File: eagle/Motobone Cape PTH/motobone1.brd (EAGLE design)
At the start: 87.3 x 54.6 mm, 23 parts, among them J1 COMPUTER-PERIPHERAL-POWERRA

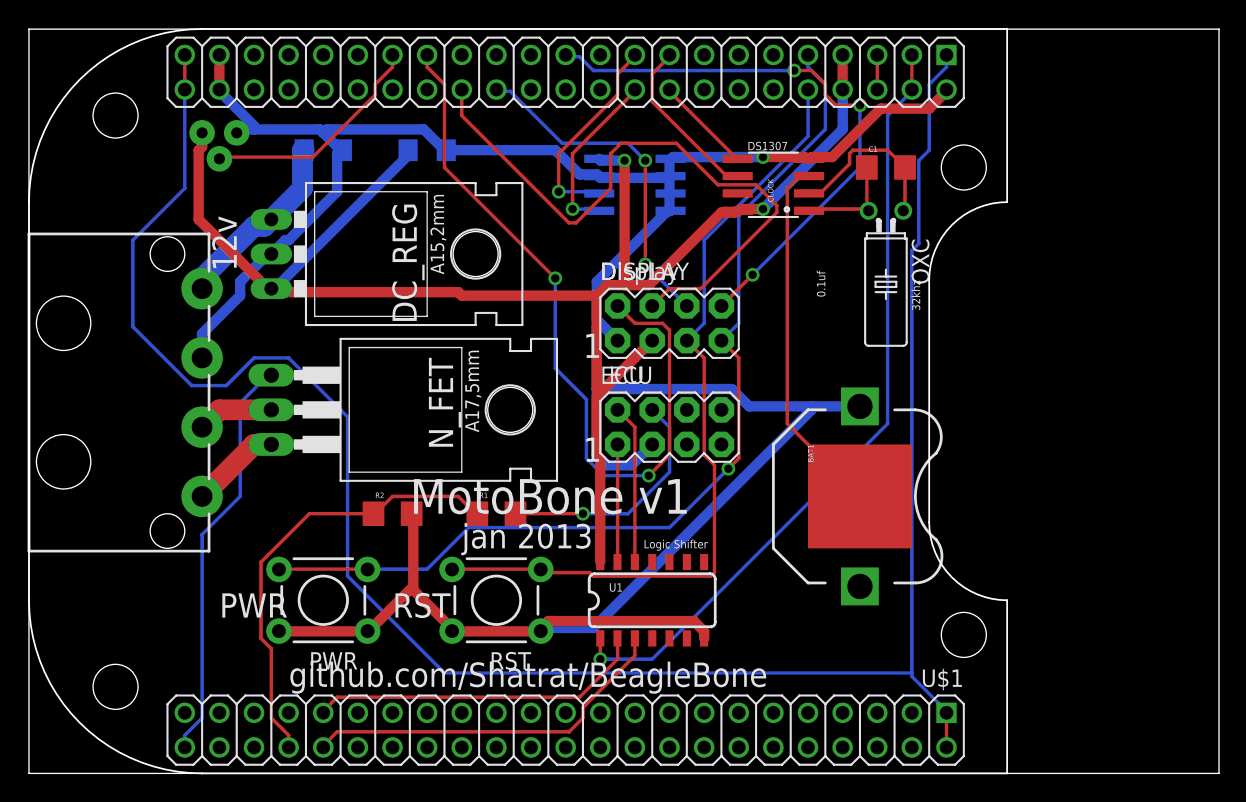
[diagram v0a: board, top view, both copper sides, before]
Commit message: updating Eagle files
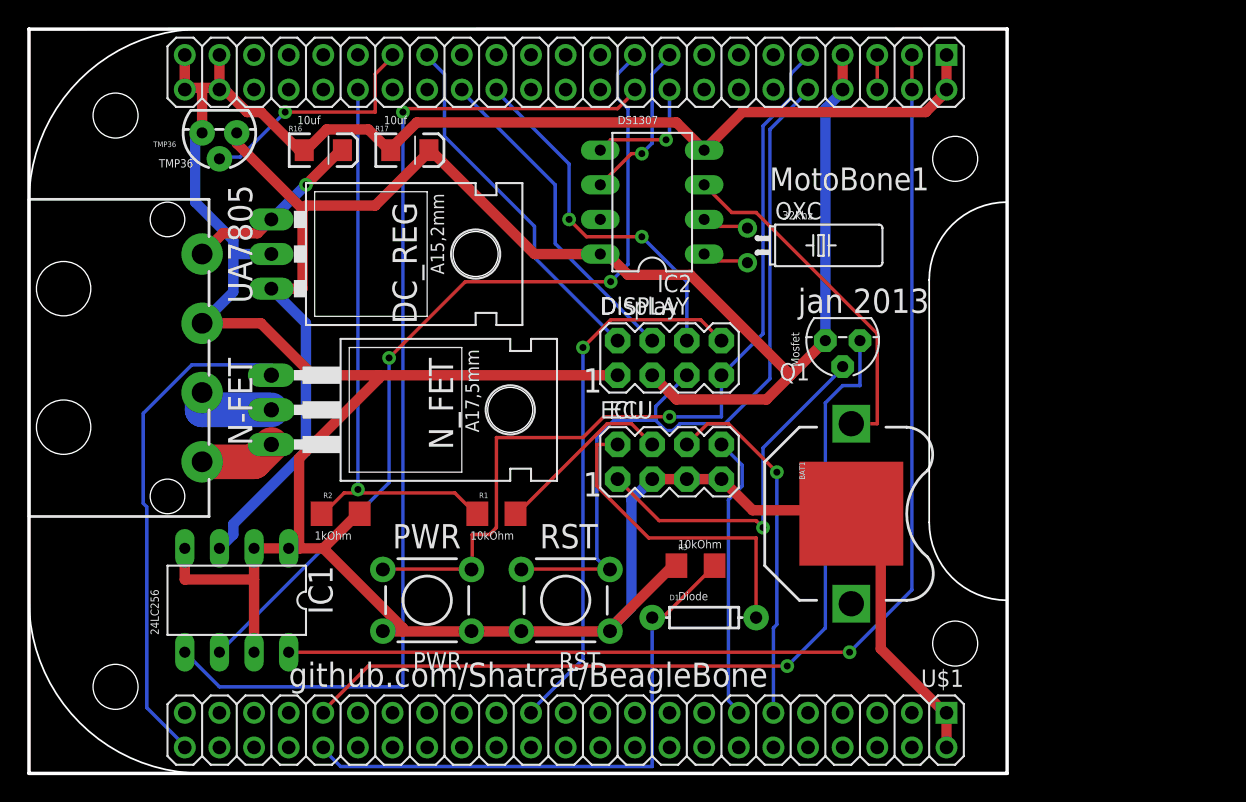
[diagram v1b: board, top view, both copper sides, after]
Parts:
- removed C1: 0.1uF, SparkFun-Capacitors:1206
- removed CLOCK: DS1307SO8, SparkFun-FreqCtrl:SO08
- removed EEPROM: EEPROM-I2CSMD, SparkFun-DigitalIC:SO08
- removed U1: (no value), SparkFun-DigitalIC:SO14
- added D1: (no value), SparkFun-DiscreteSemi:DIODE-1N4148
- added IC1: 24LC256P, microchip:DIL8
- added IC2: DS1307, adafruit:DIL08
- added Q1: FQN1N50C, adafruit:TO92
- added R3: 10k, SparkFun-Resistors:1206
- BAT1: value (none) -> 3v
- R2: value 3k -> 1k
- moved OXC 10.5 mm to (52.7, 38.7), turned to 270 degrees
- moved PWR 7.62 mm to (29.2, 12.7)
- moved RST 5.08 mm to (39.4, 12.7)
- moved R2 3.81 mm to (22.9, 19.1)
- moved DISPLAY 2.54 mm to (47.0, 30.5)
- moved ECU 2.54 mm to (47.0, 22.9)
- moved J1 2.54 mm to (10.2, 30.5)
- moved BAT1 1.42 mm to (60.3, 19.1)
- moved R17 1.27 mm to (27.9, 45.7), flipped to the top
- moved STANDOFF2 0.90 mm to (67.9, 9.53)
- moved STANDOFF3 0.90 mm to (67.9, 45.1)
- flipped R16 to the top
- flipped TMP36 to the top
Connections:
- removed net N$23: ECU.1, U1.13
- new net N$13: ECU.6, U$1.11
- new net N$14: ECU.8, U$1.13
- net GND: now also BAT1.GND, ECU.5, ECU.7, IC1.1, IC1.2, IC1.4, IC1.7, IC2.4, R3.1, U$1.1, U$1.2, U$1.47, U$1.91, U$1.92; no longer BAT1.VCC@1, CLOCK.4, EEPROM.1, EEPROM.2, EEPROM.3, EEPROM.4, EEPROM.7, U1.7
- net N$10: now also IC1.5; no longer EEPROM.5
- net N$12: now also Q1.1, U$1.37; no longer U$1.1, U$1.2, U$1.47, U$1.91, U$1.92
- net N$17: now also U$1.82; no longer U$1.40
- net N$2: now also IC2.6; no longer CLOCK.6
- net N$22: now also U$1.25; no longer U$1.69
- net N$24: now also D1.C; no longer U1.12
- net N$25: now also D1.A, R3.2; no longer U1.3
- net N$26: now also ECU.1, Q1.2; no longer U$1.37, U1.2
- net N$5: now also IC2.2; no longer C1.2, CLOCK.2
- net N$6: now also IC2.1; no longer C1.1, CLOCK.1
- net N$7: now also IC2.5; no longer CLOCK.5
- net N$8: now also BAT1.VCC@1, IC2.3; no longer BAT1.GND, CLOCK.3
- net N$9: now also IC1.6; no longer EEPROM.6
- net SYS_5V: now also IC1.3, IC2.8, Q1.3; no longer CLOCK.8, EEPROM.8, U1.14
- net VDD_3V3: now also IC1.8; no longer U1.1
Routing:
- net N$12: track 150.6 -> 62.4 mm, vias 0 -> 1
- net N$10: track 12.7 -> 77.0 mm
- net N$9: track 15.4 -> 63.3 mm, vias 1 -> 2
- net GND: track 203.0 -> 245.4 mm, vias 1 -> 0
- net VDD_3V3: track 57.5 -> 86.9 mm
- net N$3: track 55.4 -> 26.7 mm, vias 2 -> 0
- net N$13: track 0.00 -> 26.5 mm, vias 0 -> 1
- net N$1: track 46.6 -> 24.2 mm
- net N$14: track 0.00 -> 21.1 mm
- net N$25: track 27.4 -> 41.9 mm
- net N$24: track 11.7 -> 23.7 mm
- net N$17: track 32.8 -> 42.3 mm, vias 0 -> 1
- net N$5: track 12.5 -> 3.44 mm
- net N$23: track 8.63 -> 0.00 mm
- net HEAT_GPIO: track 30.1 -> 37.4 mm
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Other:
- board size 87.3 x 54.6 mm -> 71.8 x 54.6 mm
- board text added: "10kOhm"
- board text added: "10uf"
- board text added: "1kOhm"
- board text added: "24LC256"
- board text added: "Diode"
- board text added: "Mosfet"
- board text added: "MotoBone1"
- board text added: "N-FET"
- board text added: "TMP36"
- board text added: "UA7805"
- board text removed: "0.1uf"
- board text removed: "12v"
- board text removed: "Logic Shifter"
- board text removed: "MotoBone v1"
